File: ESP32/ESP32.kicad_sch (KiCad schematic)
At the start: 4 parts, among them Q1 Q_NPN_EBC, U2 Generic_5v_Module

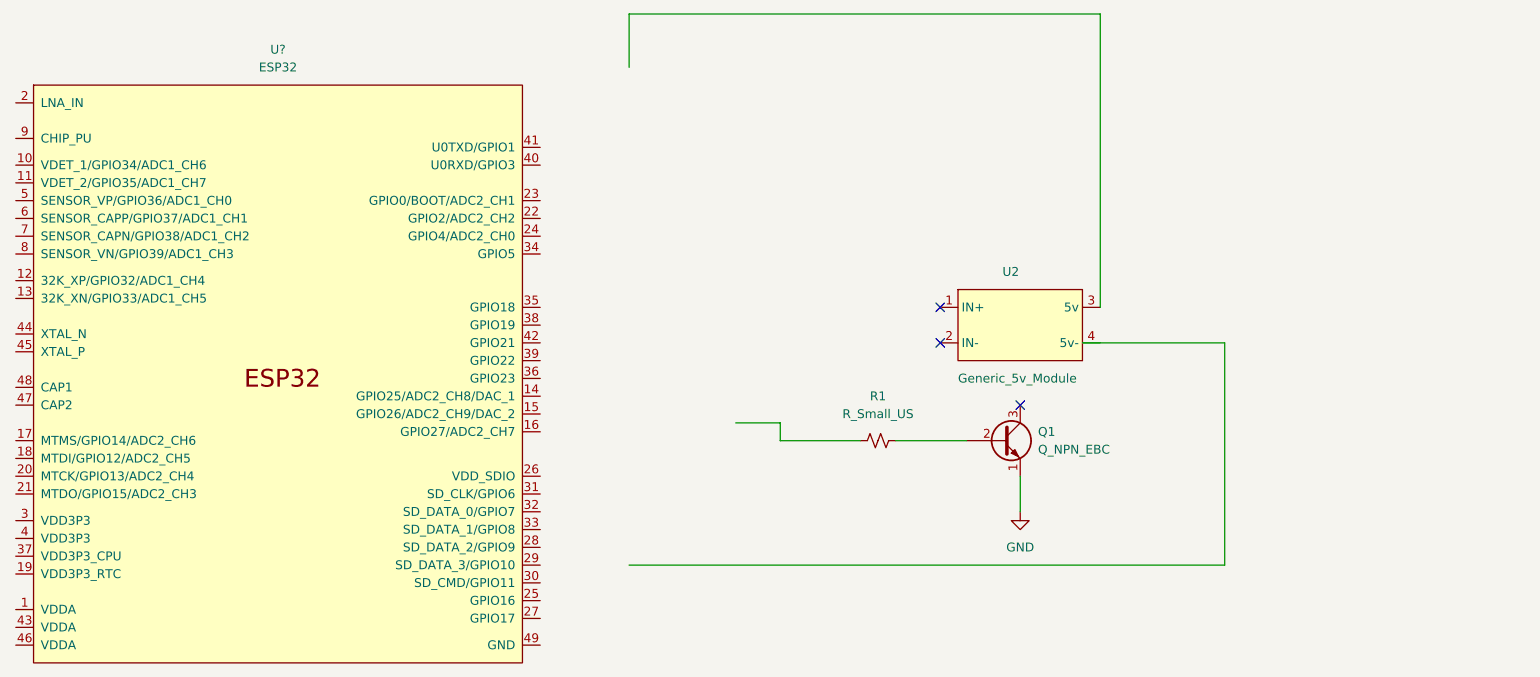
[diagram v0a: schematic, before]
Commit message: KiCad Changes.
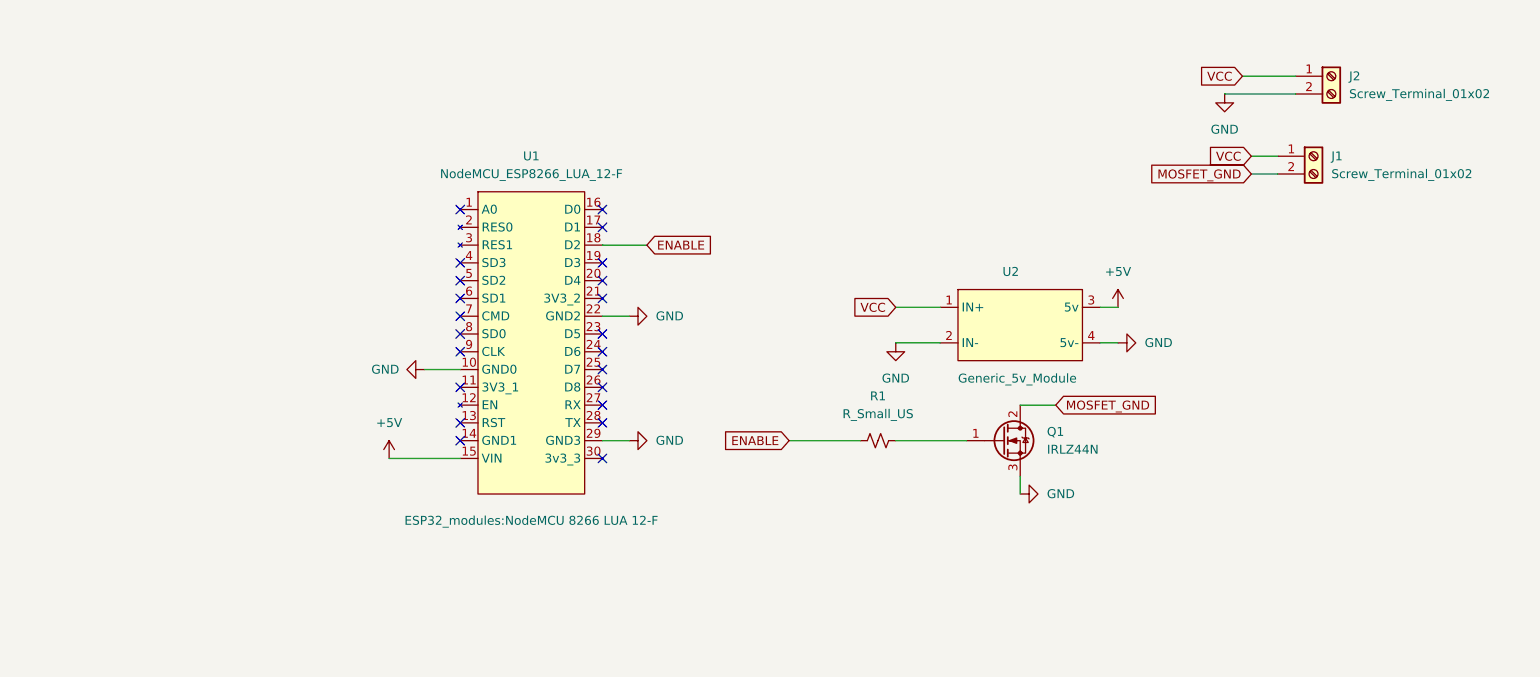
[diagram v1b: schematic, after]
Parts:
- removed Q1: Q_NPN_EBC, symbol Device:Q_NPN_EBC
- removed U?: ESP32, ESP32_modules:ESP32-DevKitC, symbol Espressif:ESP32
- added J1, J2: Screw_Terminal_01x02, TerminalBlock:TerminalBlock_bornier-2_P5.08mm, symbol Connector:Screw_Terminal_01x02
- added Q1: IRLZ44N, Package_TO_SOT_THT:TO-220-3_Vertical, symbol Transistor_FET:IRLZ44N
- added U1: NodeMCU_ESP8266_LUA_12-F, ESP32_modules:NodeMCU 8266 LUA 12-F, symbol Espressif:NodeMCU_ESP8266_LUA_12-F
- R1: footprint (none) -> Resistor_THT:R_Axial_DIN0207_L6.3mm_D2.5mm_P5.08mm_Vertical
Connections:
- net GND: now also U2.2 (IN-), U2.4 (5v-), J2.2 (Pin_2), Q1.3 (S), U1.10 (GND0), U1.22 (GND2), U1.29 (GND3)
- net at R1.2: now also Q1.1 (G)
- net VCC: now reaches U2.1 (IN+)
- net VCC: now also J1.1 (Pin_1), J2.1 (Pin_1)
- net +5V: now reaches U2.3 (5v)
- net +5V: now also U1.15 (VIN)
- net ENABLE: now reaches R1.1
- net ENABLE: now also U1.18 (D2)
- new net MOSFET_GND: J1.2 (Pin_2), Q1.2 (D)
- no-connect marks 3 -> 22
